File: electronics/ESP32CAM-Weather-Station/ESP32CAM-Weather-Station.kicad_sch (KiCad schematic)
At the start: 96 parts, among them IC1 BME688, IC2 SGP41-D-R4, IC3 VEML7700-TT, IC4 BQ24093DGQR, IC5 BQ29707DSET, IC6 MCP3426A0T-E_SN, IC7 TPS63070RNMR, J1 B4B-PH-SM4-TB_LF__SN_, J10 Conn_01x02_Pin, J2 B4B-PH-SM4-TB_LF__SN_, J3 B4B-PH-SM4-TB_LF__SN_, J4 B4B-PH-SM4-TB_LF__SN_, J5 B4B-PH-SM4-TB_LF__SN_, J6 XT30UPB-M, J7 Conn_01x02_Pin, J8 Conn_01x02_Pin, J9 Conn_01x02_Pin, Q1 SIHLL110TR-GE3, Q2 CSD16406Q3, Q3 CSD16406Q3, U1 ESP32-CAM, U2 TPS631000DRLR, U3 GDT25-07-S1-RP

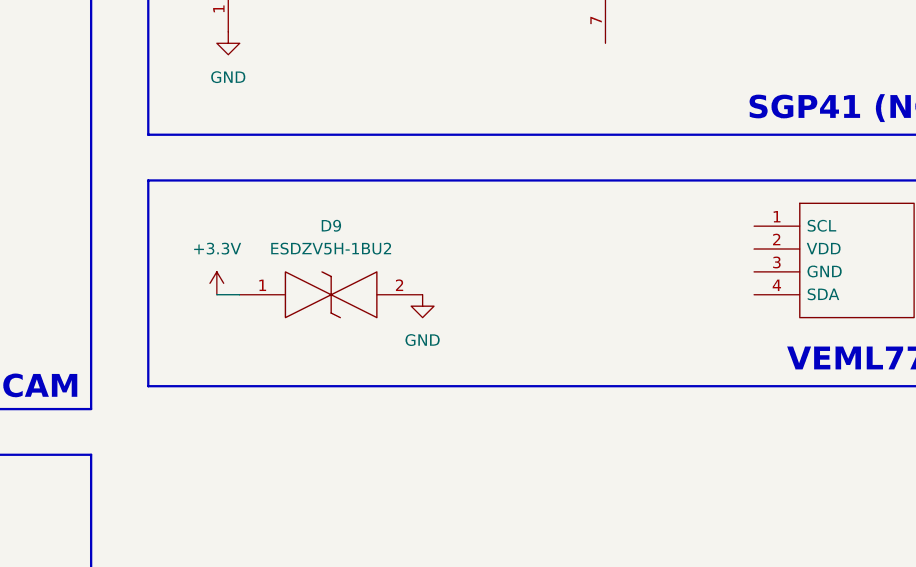
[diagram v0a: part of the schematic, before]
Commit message: [WIP] Routed light sensor.
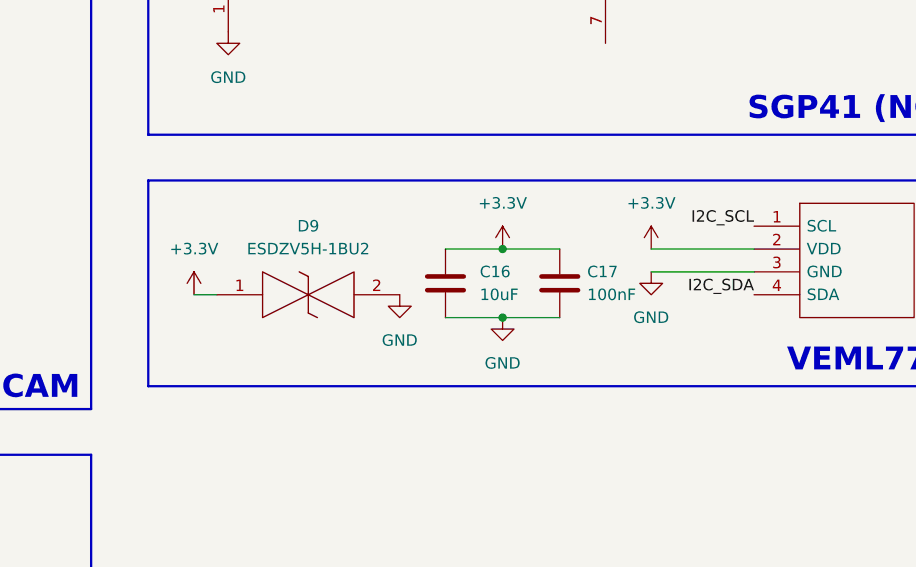
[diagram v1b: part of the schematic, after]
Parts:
- added C16: 10uF, Capacitor_SMD:C_0805_2012Metric_Pad1.18x1.45mm_HandSolder, symbol Device:C
- added C17: 100nF, Capacitor_SMD:C_0603_1608Metric_Pad1.08x0.95mm_HandSolder, symbol Device:C
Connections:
- net +3.3V: now also IC3.2 (VDD), C16.1, C17.2
- net GND: now also IC3.3 (GND), C16.2, C17.1
- net I2C_SCL: now also IC3.1 (SCL)
- net I2C_SDA: now also IC3.4 (SDA)
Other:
- moved on the sheet: D9
